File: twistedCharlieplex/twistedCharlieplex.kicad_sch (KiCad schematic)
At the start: 1 part, among them U2 STM32L412CBUxP

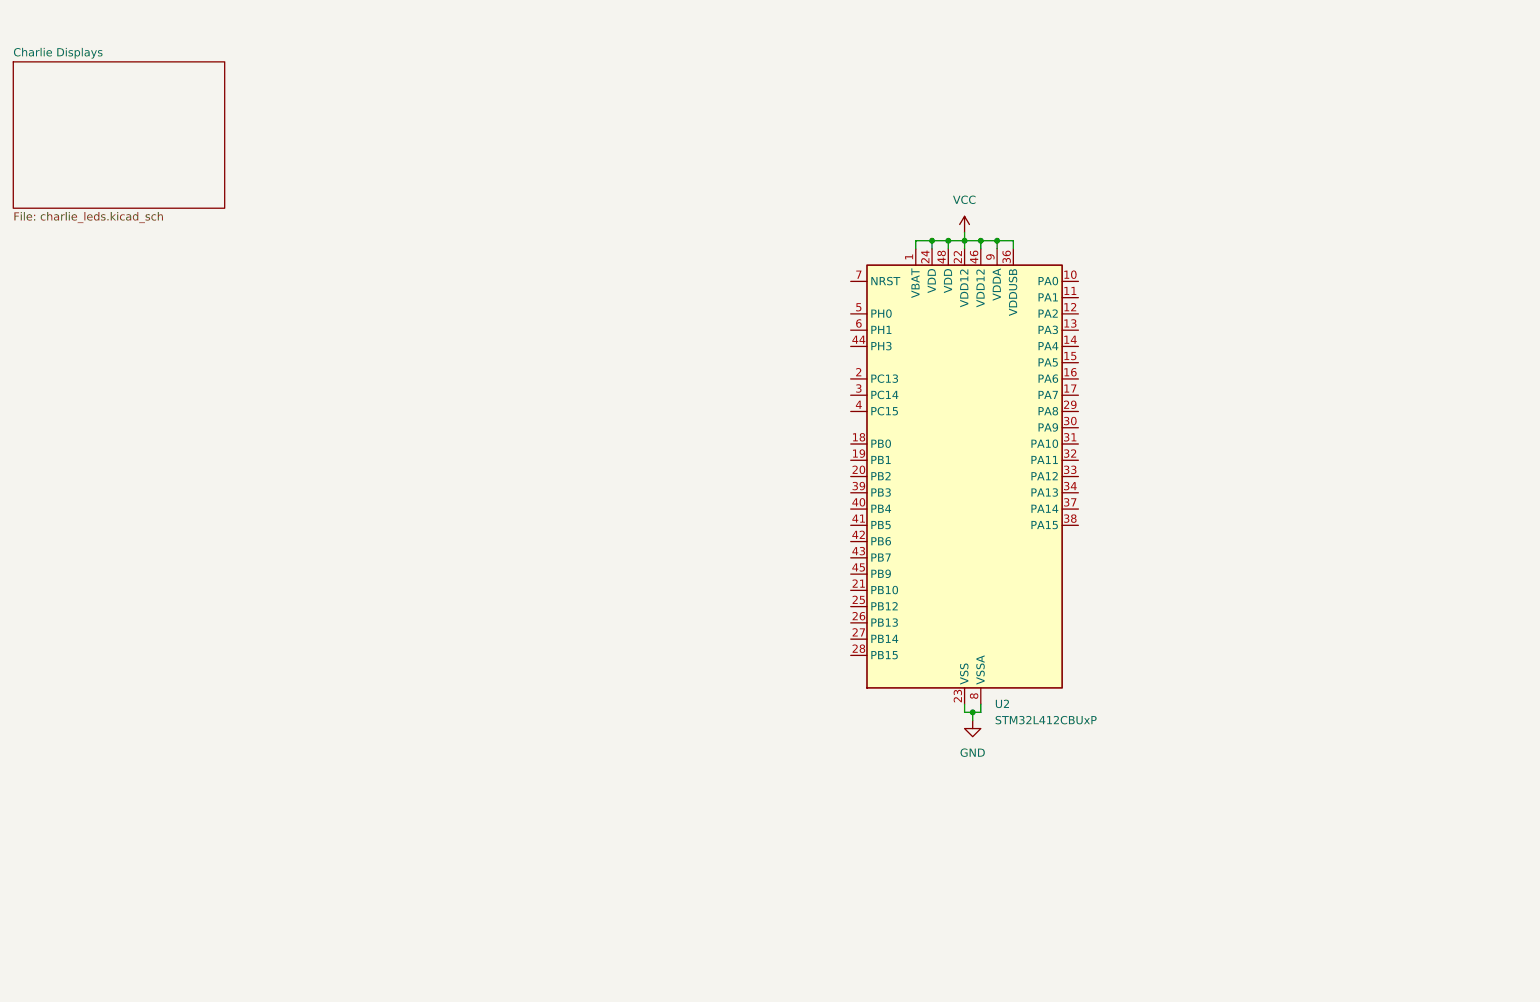
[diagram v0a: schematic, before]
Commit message: spirograph layout. let the nightmares begin
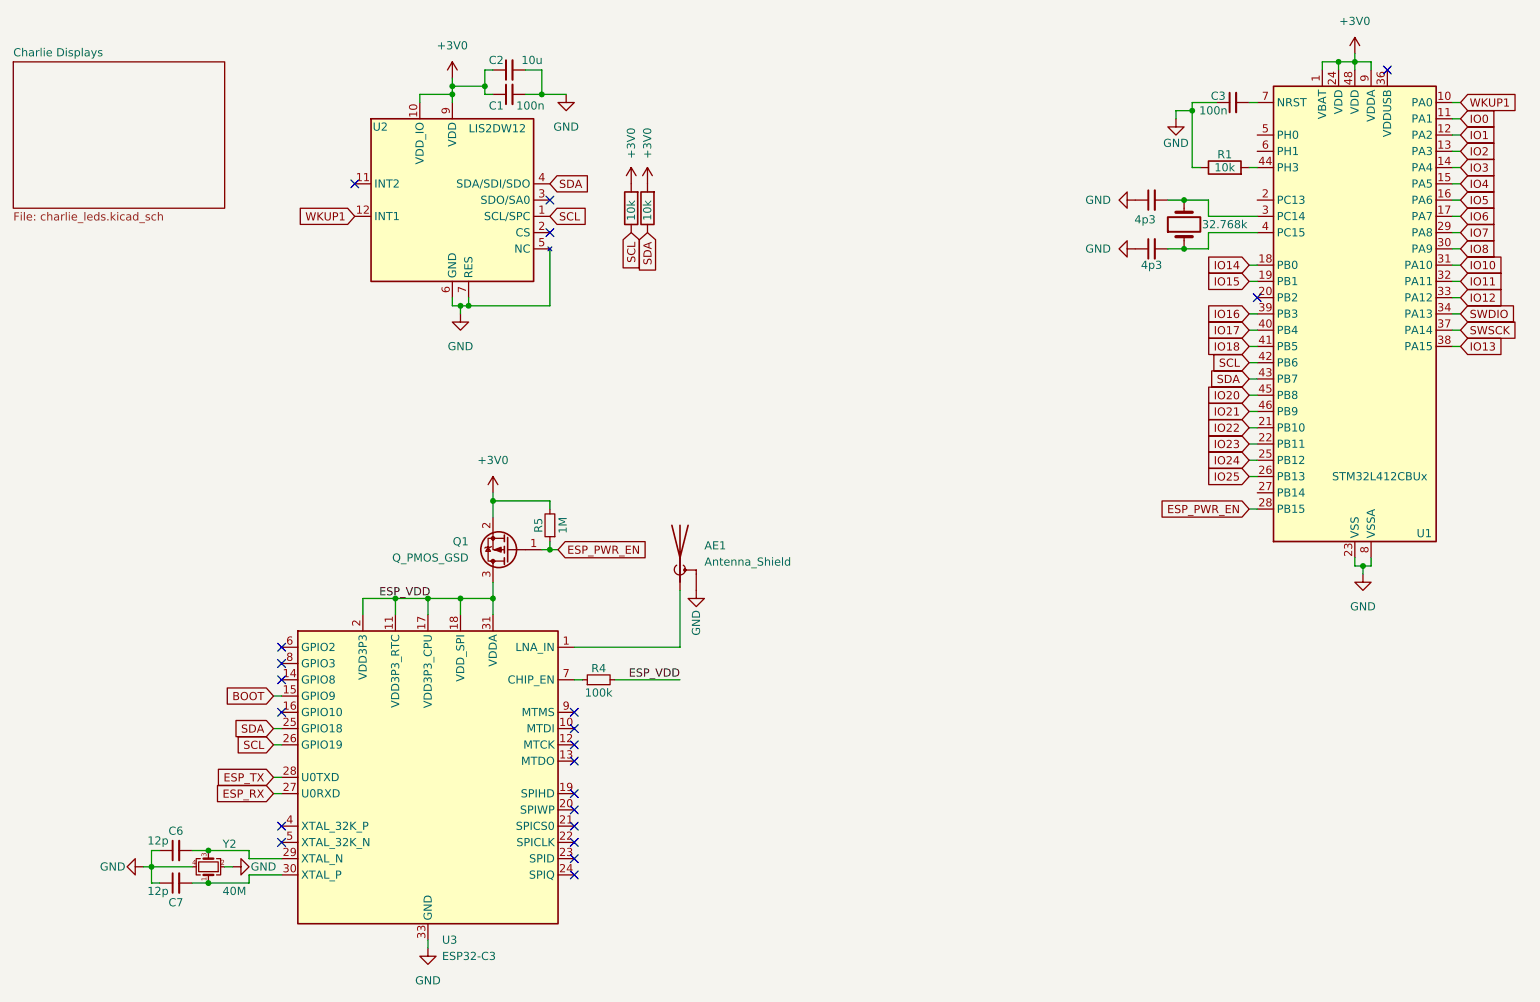
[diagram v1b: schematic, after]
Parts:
- removed U2: STM32L412CBUxP, Package_DFN_QFN:QFN-48-1EP_7x7mm_P0.5mm_EP5.6x5.6mm, symbol MCU_ST_STM32L4:STM32L412CBUxP
- added AE1: Antenna_Shield, Antenna_SMD:C209892, symbol Device:Antenna_Shield
- added C1, C3: 100n, Capacitor_SMD:C_0402_1005Metric, symbol Device:C_Small
- added C2: 10u, Capacitor_SMD:C_0402_1005Metric, symbol Device:C_Small
- added C4, C5: 4p3, Capacitor_SMD:C_0402_1005Metric, symbol Device:C_Small
- added C6, C7: 12p, Capacitor_SMD:C_0402_1005Metric, symbol Device:C_Small
- added Q1: Q_PMOS_GSD, Package_TO_SOT_SMD:SOT-523, symbol Device:Q_PMOS_GSD
- added R1, R2, R3: 10k, Resistor_SMD:R_0402_1005Metric, symbol Device:R
- added R4: 100k, Resistor_SMD:R_0402_1005Metric, symbol Device:R_Small
- added R5: 1M, Resistor_SMD:R_0402_1005Metric, symbol Device:R_Small
- added U1: STM32L412CBUx, Package_DFN_QFN:QFN-48-1EP_7x7mm_P0.5mm_EP5.6x5.6mm, symbol MCU_ST_STM32L4:STM32L412CBUx
- added U2: LIS2DW12, Package_LGA:LGA-12_2x2mm_P0.5mm, symbol Sensor_IMU:LIS2DW12
- added U3: ESP32-C3, Package_DFN_QFN:QFN-32-1EP_5x5mm_P0.5mm_EP3.7x3.7mm, symbol MCU_Espressif:ESP32-C3
- added Y1: 32.768k, Crystal:Crystal_SMD_3215-2Pin_3.2x1.5mm, symbol Device:Crystal
- added Y2: 40M, SMD_Crystal:Crystal_SMD_1612_4P, symbol Device:Crystal_GND24_Small
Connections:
- net GND: now also AE1.2 (Shield), C1.2, C2.2, C3.1, C4.1, C5.1, C6.1, C7.1, R1.1, U1.23 (VSS), U1.35 (VSS), U1.47 (VSS), U1.49 (VSS), U1.8 (VSSA), U2.5 (NC), U2.6 (GND), U2.7 (RES), U2.8 (GND), U3.33 (GND), Y2.2, Y2.4
- new net: AE1.1 (A), U3.1 (LNA_IN)
- new net: C6.2, U3.29 (XTAL_N), Y2.3
- new net: C7.2, U3.30 (XTAL_P), Y2.1
- new net: R4.1, U3.7 (CHIP_EN)
- new net: C5.2, U1.4 (PC15), Y1.1
- new net: C4.2, U1.3 (PC14), Y1.2
- new net: C3.2, U1.7 (NRST)
- new net: R1.2, U1.44 (PH3)
- new net +3V0: C1.1, C2.1, Q1.2 (S), R2.2, R3.2, R5.2, U1.1 (VBAT), U1.24 (VDD), U1.48 (VDD), U1.9 (VDDA), U2.10 (VDD_IO), U2.9 (VDD)
- new net BOOT: U3.15 (GPIO9)
- new net ESP_PWR_EN: Q1.1 (G), R5.1, U1.28 (PB15)
- new net ESP_RX: U3.27 (U0RXD)
- new net ESP_TX: U3.28 (U0TXD)
- new net ESP_VDD: Q1.3 (D), R4.2, U3.11 (VDD3P3_RTC), U3.17 (VDD3P3_CPU), U3.18 (VDD_SPI), U3.2 (VDD3P3), U3.3 (VDD3P3), U3.31 (VDDA), U3.32 (VDDA)
- new net IO0: U1.11 (PA1)
- new net IO1: U1.12 (PA2)
- new net IO10: U1.31 (PA10)
- new net IO11: U1.32 (PA11)
- new net IO12: U1.33 (PA12)
- new net IO13: U1.38 (PA15)
- new net IO14: U1.18 (PB0)
- new net IO15: U1.19 (PB1)
- new net IO16: U1.39 (PB3)
- new net IO17: U1.40 (PB4)
- new net IO18: U1.41 (PB5)
- new net IO2: U1.13 (PA3)
- new net IO20: U1.45 (PB8)
- new net IO21: U1.46 (PB9)
- new net IO22: U1.21 (PB10)
- new net IO23: U1.22 (PB11)
- new net IO24: U1.25 (PB12)
- new net IO25: U1.26 (PB13)
- new net IO3: U1.14 (PA4)
- new net IO4: U1.15 (PA5)
- new net IO5: U1.16 (PA6)
- new net IO6: U1.17 (PA7)
- new net IO7: U1.29 (PA8)
- new net IO8: U1.30 (PA9)
- new net SCL: R2.1, U1.42 (PB6), U2.1 (SCL/SPC), U3.26 (GPIO19)
- new net SDA: R3.1, U1.43 (PB7), U2.4 (SDA/SDI/SDO), U3.25 (GPIO18)
- new net SWDIO: U1.34 (PA13)
- new net SWSCK: U1.37 (PA14)
- new net WKUP1: U1.10 (PA0), U2.12 (INT1)
- no-connect marks 0 -> 21
